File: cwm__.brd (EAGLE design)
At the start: 50 x 42.9 mm, 83 parts, among them U1 STM32L476, U2 24AA64T, U3 LSM9DS0, U4 MS5803-14BA, U5 MX25L25635F, U6 RN4020, U7 LTR-303ALS, U8 LM393, U9 MK3200, X1 ABS06-32.768KHZ-9-1-T

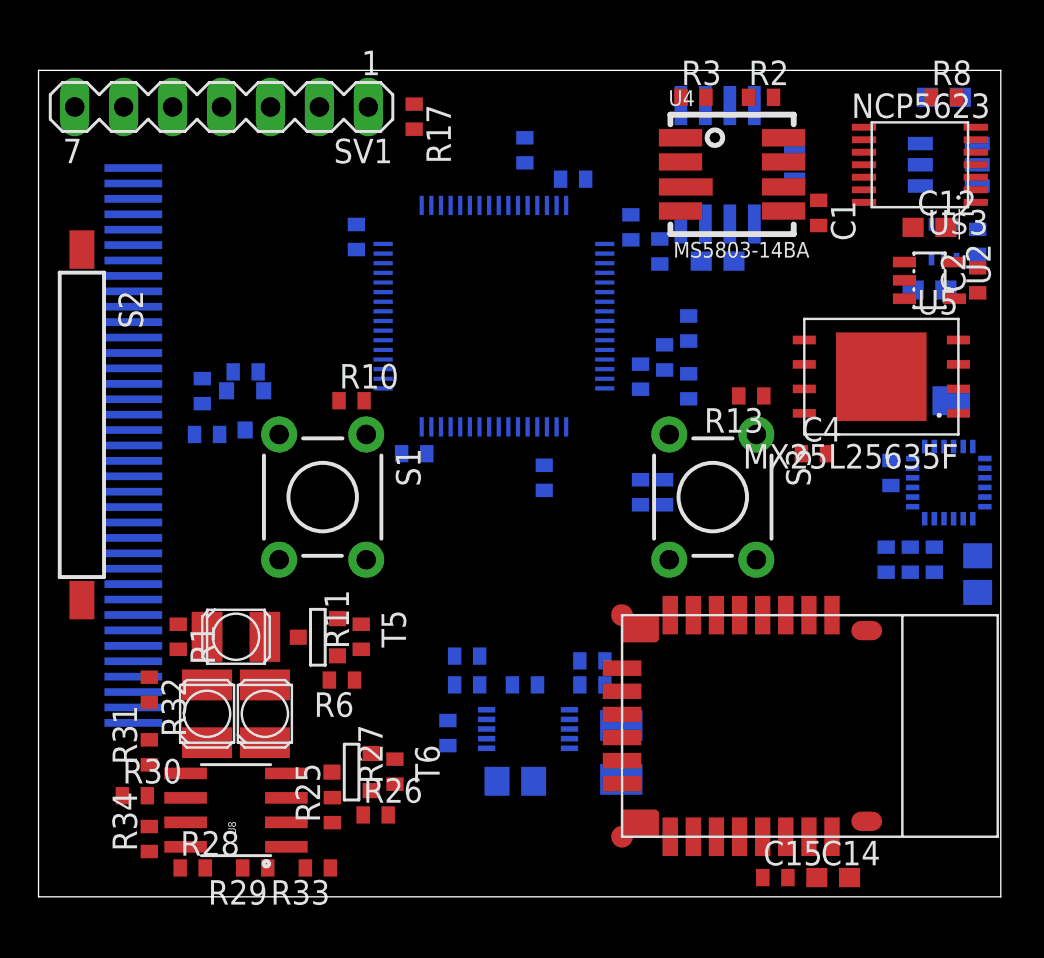
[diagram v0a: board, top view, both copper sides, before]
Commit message: routed version 0.1a
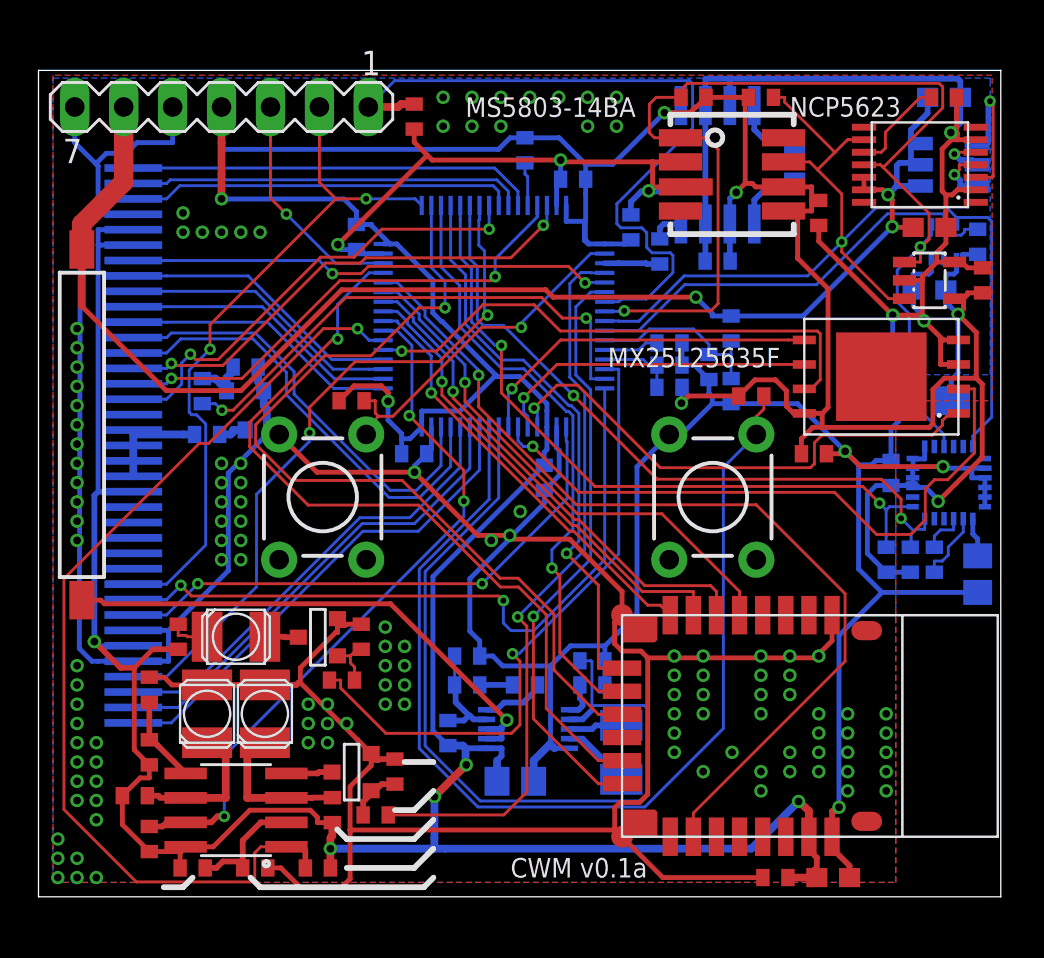
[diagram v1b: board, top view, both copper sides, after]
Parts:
- C13: device resistor:C0603 -> resistor:C0402
- T4: value (none) -> BSR202N L6327
- moved R18 7.75 mm to (32.8, 28.8), turned to 180 degrees
- moved R36 5.65 mm to (32.8, 26.4), turned to 0 degrees
- moved C10 2.35 mm to (34.8, 27.5)
- moved R38 2.21 mm to (36.0, 26.2)
- moved R37 2.20 mm to (36.0, 29.5)
- moved C20 1.62 mm to (32.8, 27.6), turned to 0 degrees
- moved C2 0.25 mm to (49.0, 32.0)
- moved R12 0.25 mm to (10.8, 27.5)
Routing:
- net GND: track 0.00 -> 373.6 mm, vias 0 -> 128
- net VCC: track 0.00 -> 292.2 mm, vias 0 -> 12
- net VIN: track 0.00 -> 73.5 mm, vias 0 -> 3
- net SCL: track 0.00 -> 62.3 mm, vias 0 -> 2
- net N$25: track 0.00 -> 55.0 mm
- net SDA: track 0.00 -> 53.8 mm, vias 0 -> 1
- net N$41: track 0.00 -> 50.8 mm, vias 0 -> 1
- net N$44: track 0.00 -> 47.9 mm, vias 0 -> 1
- net N$51: track 0.00 -> 45.5 mm, vias 0 -> 1
- net N$9: track 0.00 -> 43.0 mm
- net N$45: track 0.00 -> 41.4 mm, vias 0 -> 1
- net N$39: track 0.00 -> 38.1 mm, vias 0 -> 1
- net N$35: track 0.00 -> 37.9 mm
- net N$8: track 0.00 -> 36.8 mm, vias 0 -> 2
- net N$42: track 0.00 -> 36.7 mm, vias 0 -> 3
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- added copper zone on layer 1, net GND
- added copper zone on layer 16, net GND
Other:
- board text added: "CWM v0.1a"
